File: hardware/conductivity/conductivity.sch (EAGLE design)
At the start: 18 parts, among them IC1 AD820R, U1 TLV2374IDR, U2 TLE2426CD

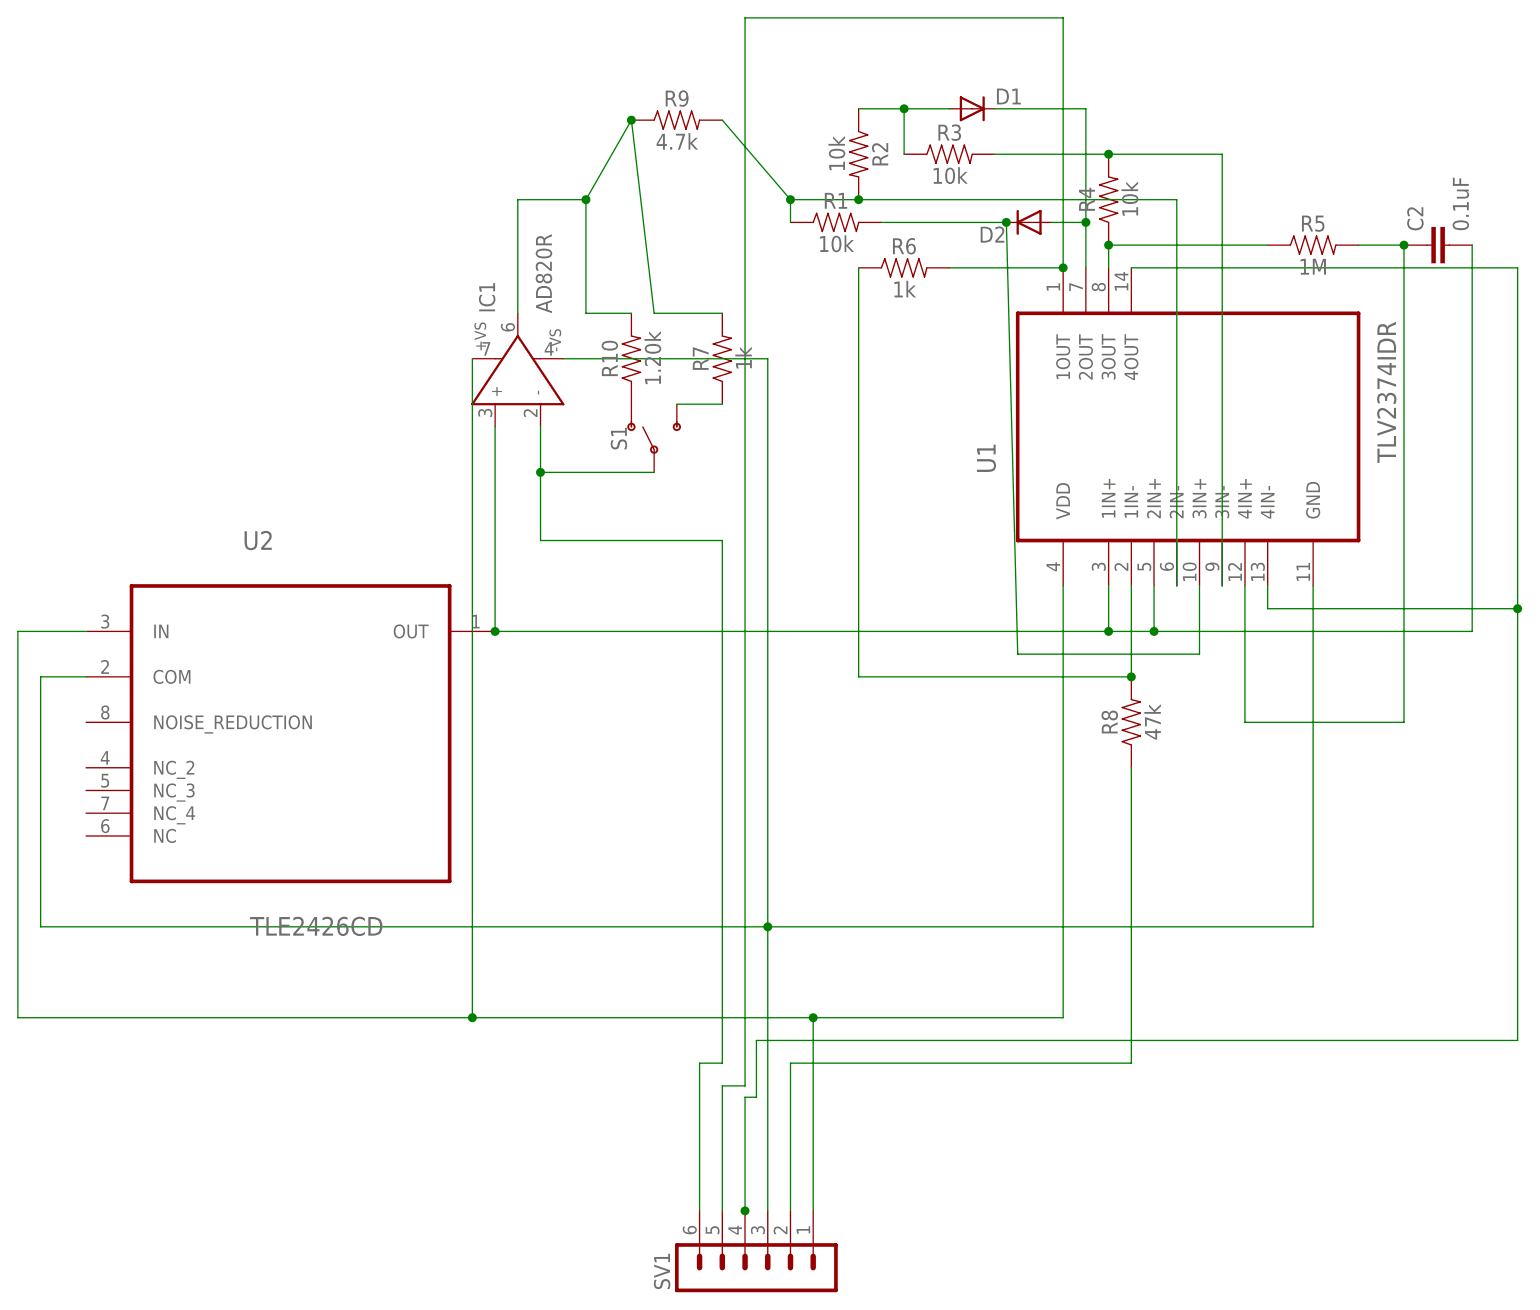
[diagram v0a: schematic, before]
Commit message: november update
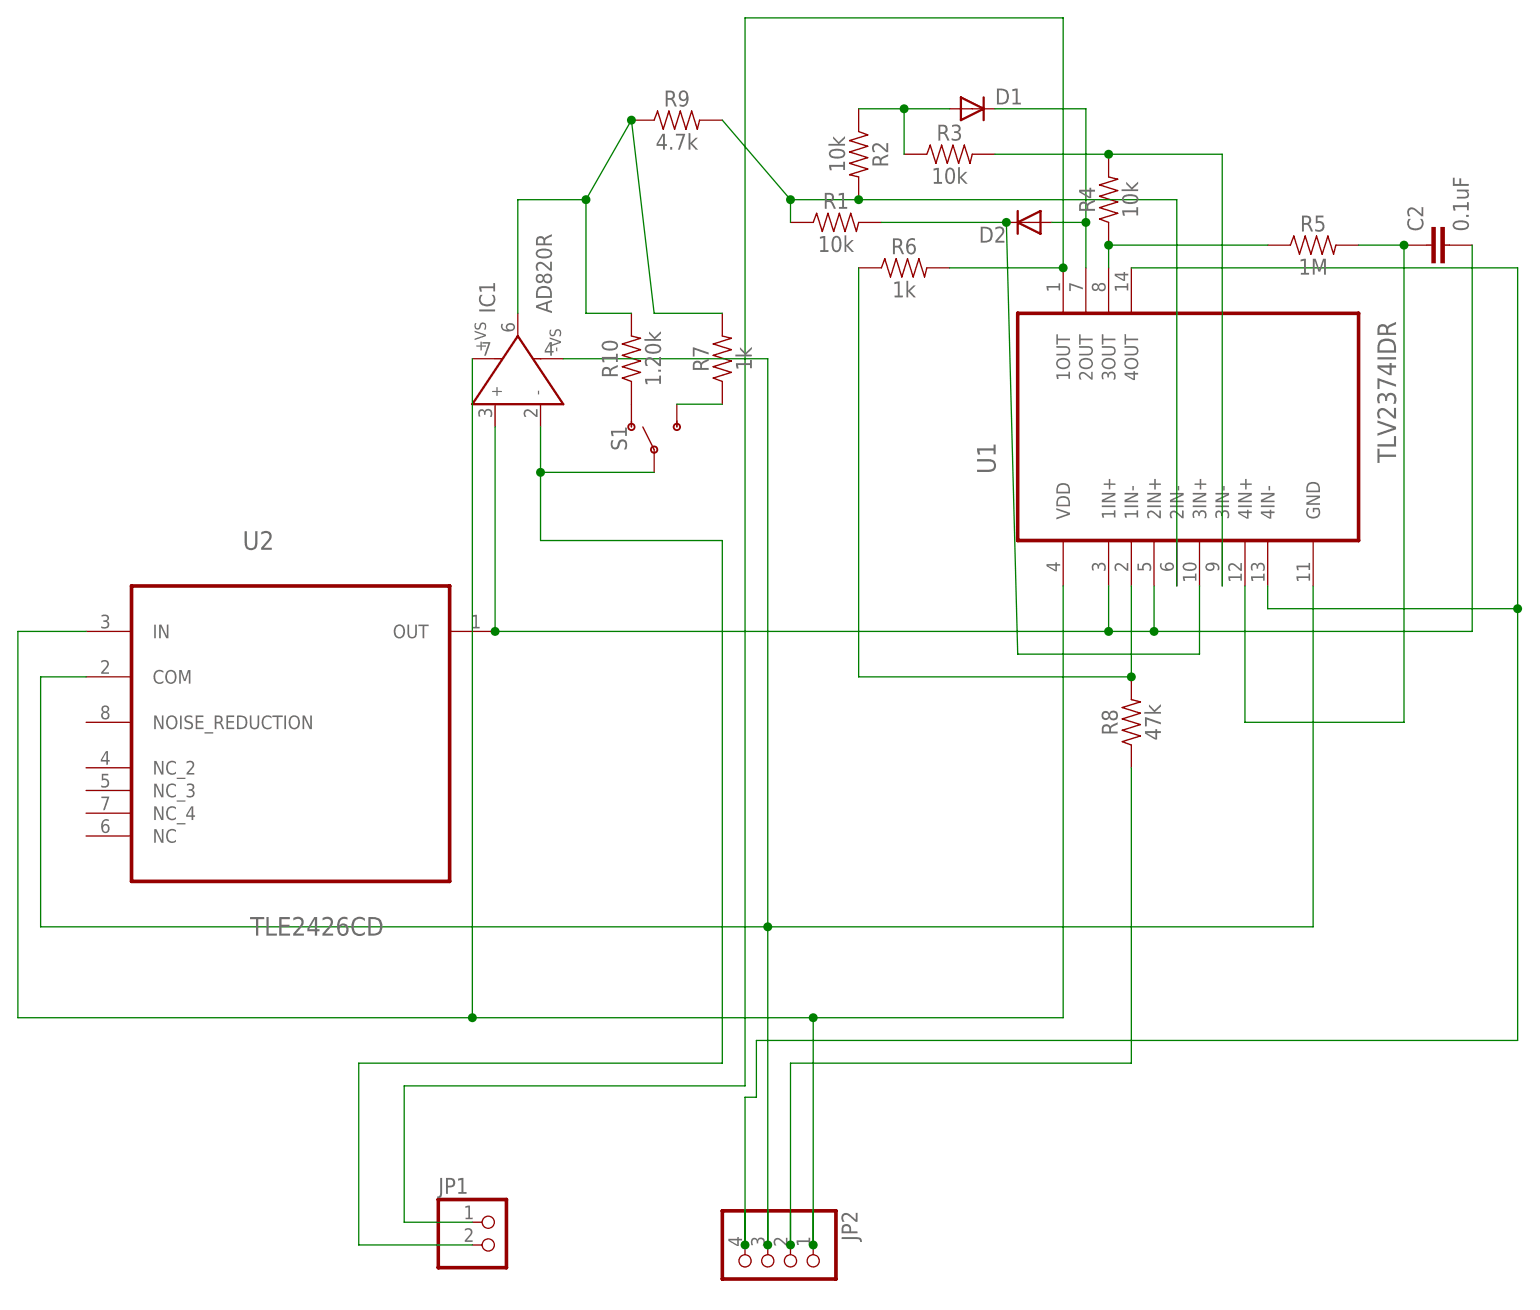
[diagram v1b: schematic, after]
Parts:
- removed SV1: (no value), con-lstb:MA06-1
- added JP1: (no value), pinhead:PINHD-1X2
- added JP2: (no value), pinhead:PINHD-1X4
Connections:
- net FROMWATER: now also JP1.2; no longer SV1.6
- net N$1: now also JP2.1; no longer SV1.1
- net N$13: now also JP2.4; no longer SV1.4
- net N$14: now also JP2.2; no longer SV1.2
- net N$15: now also JP2.3; no longer SV1.3
- net N$16: now also JP1.1; no longer SV1.5

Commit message: Revert "Updating."
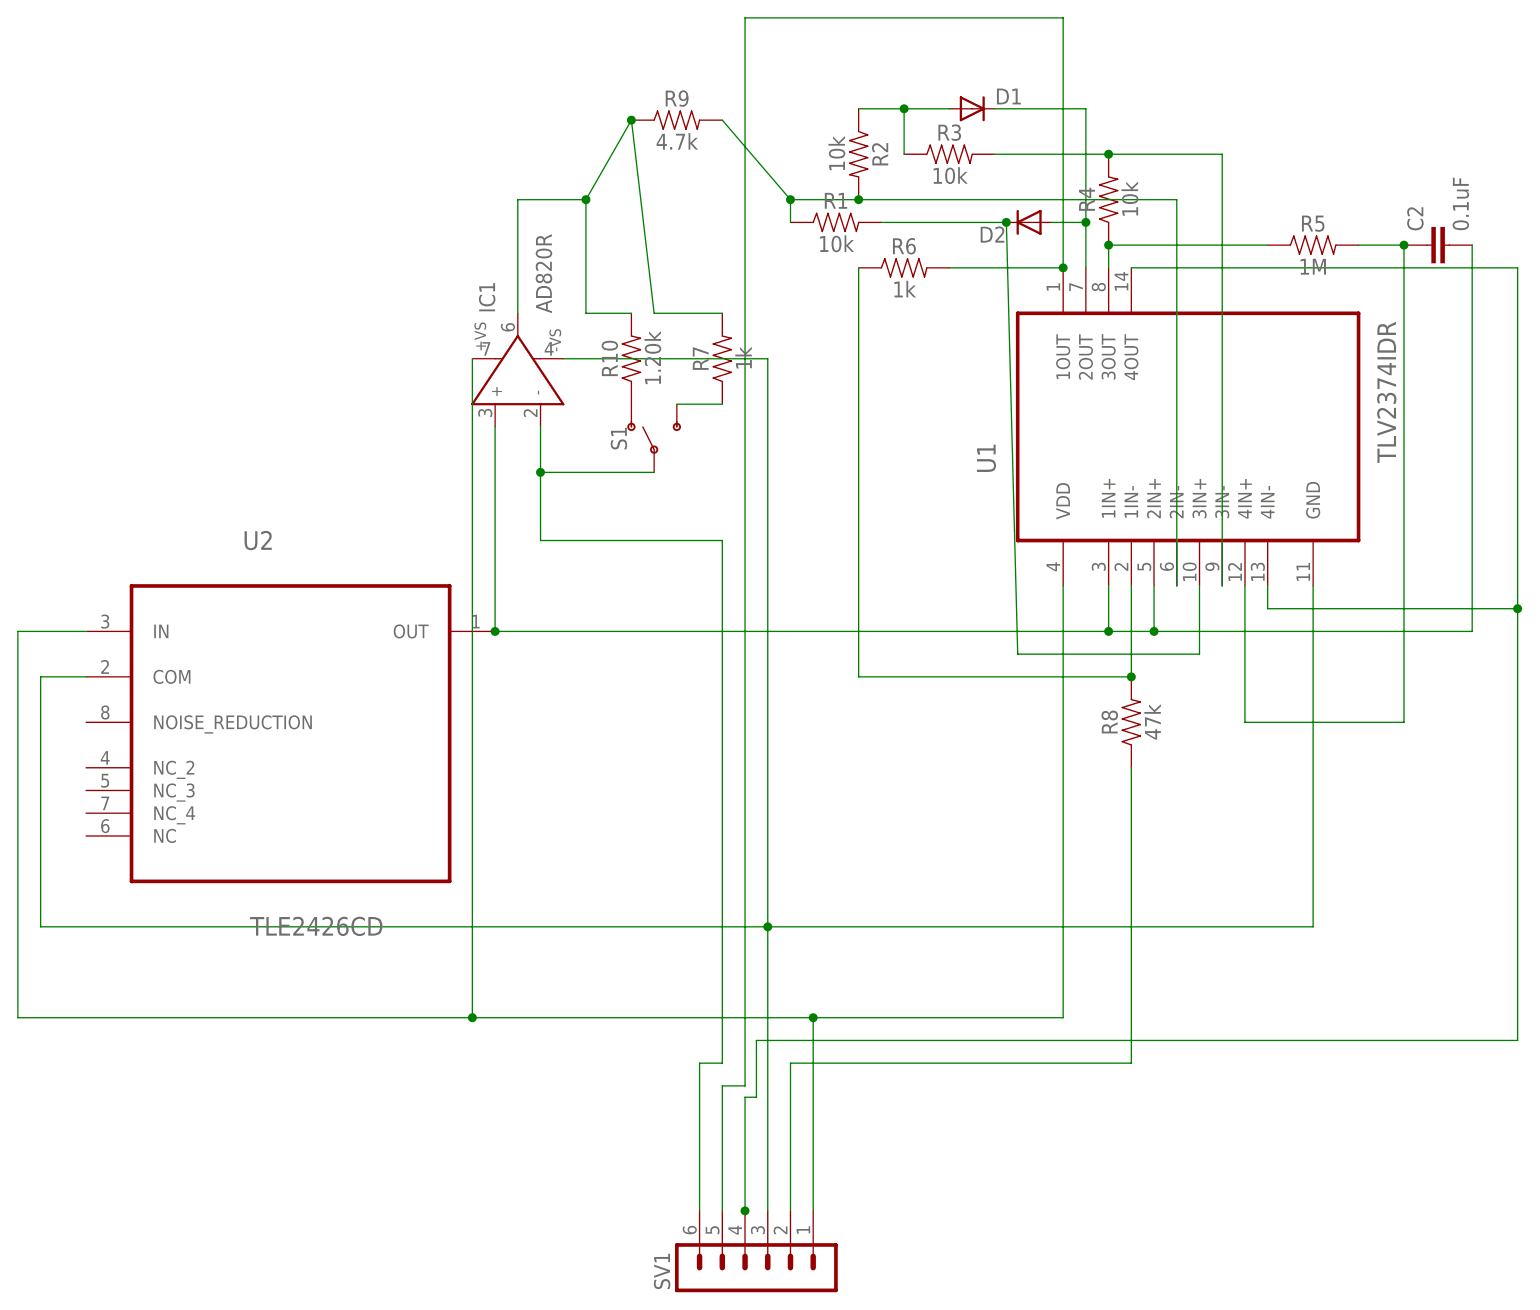
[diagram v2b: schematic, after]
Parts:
- removed JP1: (no value), pinhead:PINHD-1X2
- removed JP2: (no value), pinhead:PINHD-1X4
- added SV1: (no value), con-lstb:MA06-1
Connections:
- net FROMWATER: now also SV1.6; no longer JP1.2
- net N$1: now also SV1.1; no longer JP2.1
- net N$13: now also SV1.4; no longer JP2.4
- net N$14: now also SV1.2; no longer JP2.2
- net N$15: now also SV1.3; no longer JP2.3
- net N$16: now also SV1.5; no longer JP1.1
